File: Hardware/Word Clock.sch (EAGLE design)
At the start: 41 parts, among them IC1 MEGA32-A, IC2 HT7333, IC3 DS3231, IC4 MCP73831, J1 LiPo

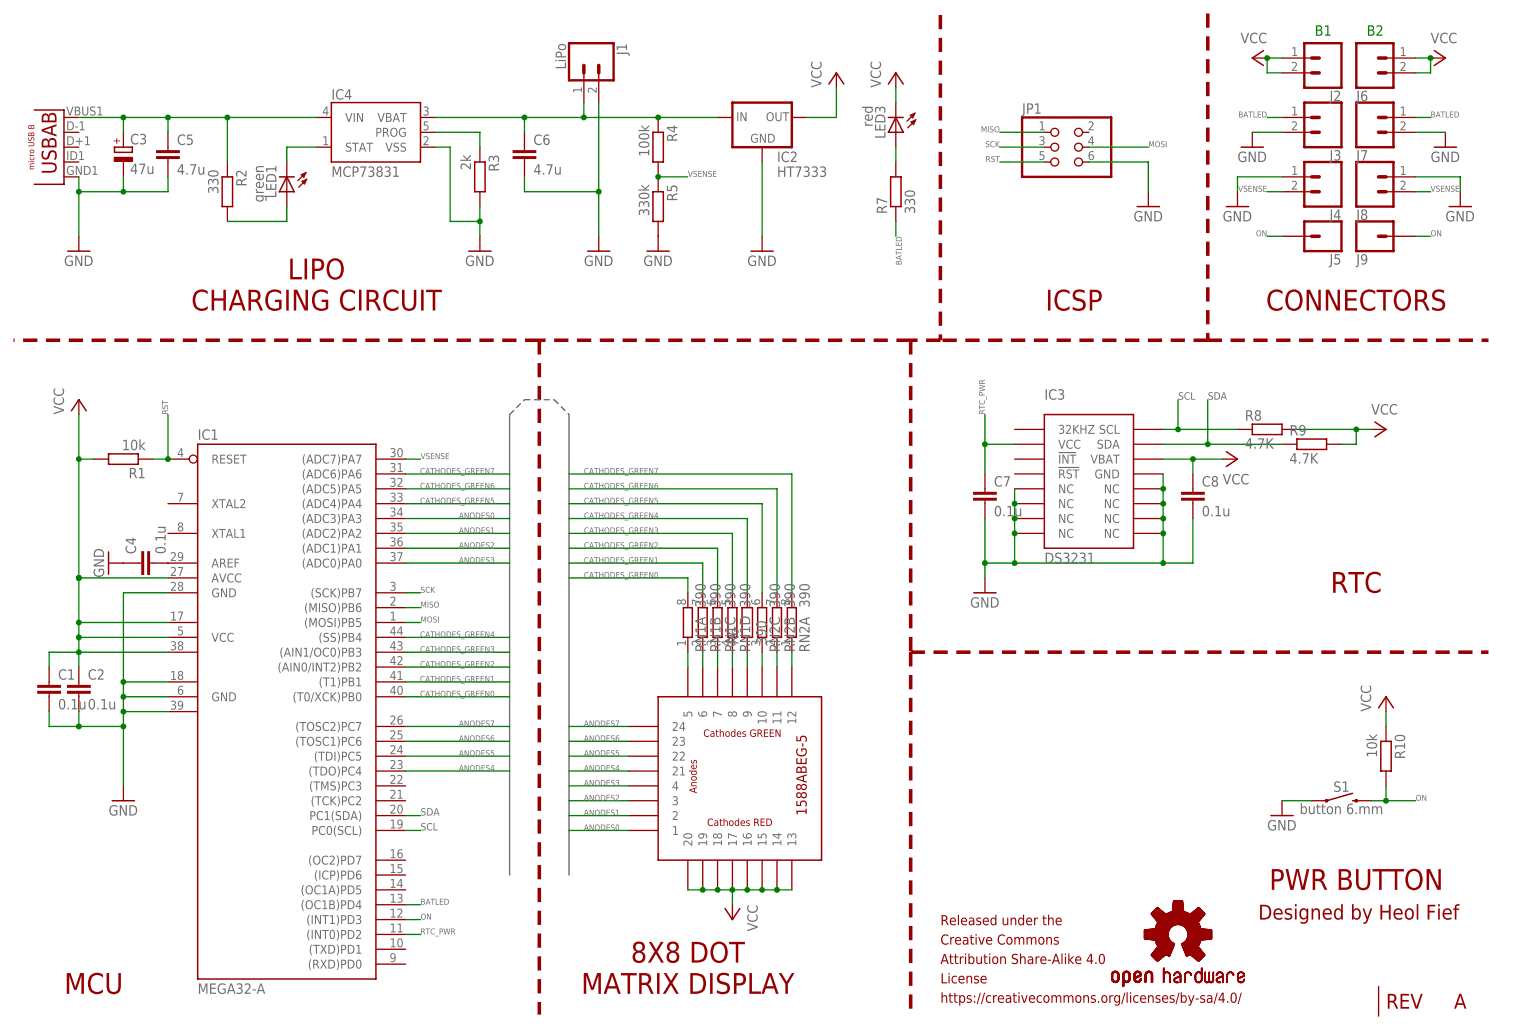
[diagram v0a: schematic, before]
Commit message: Update Eagle files
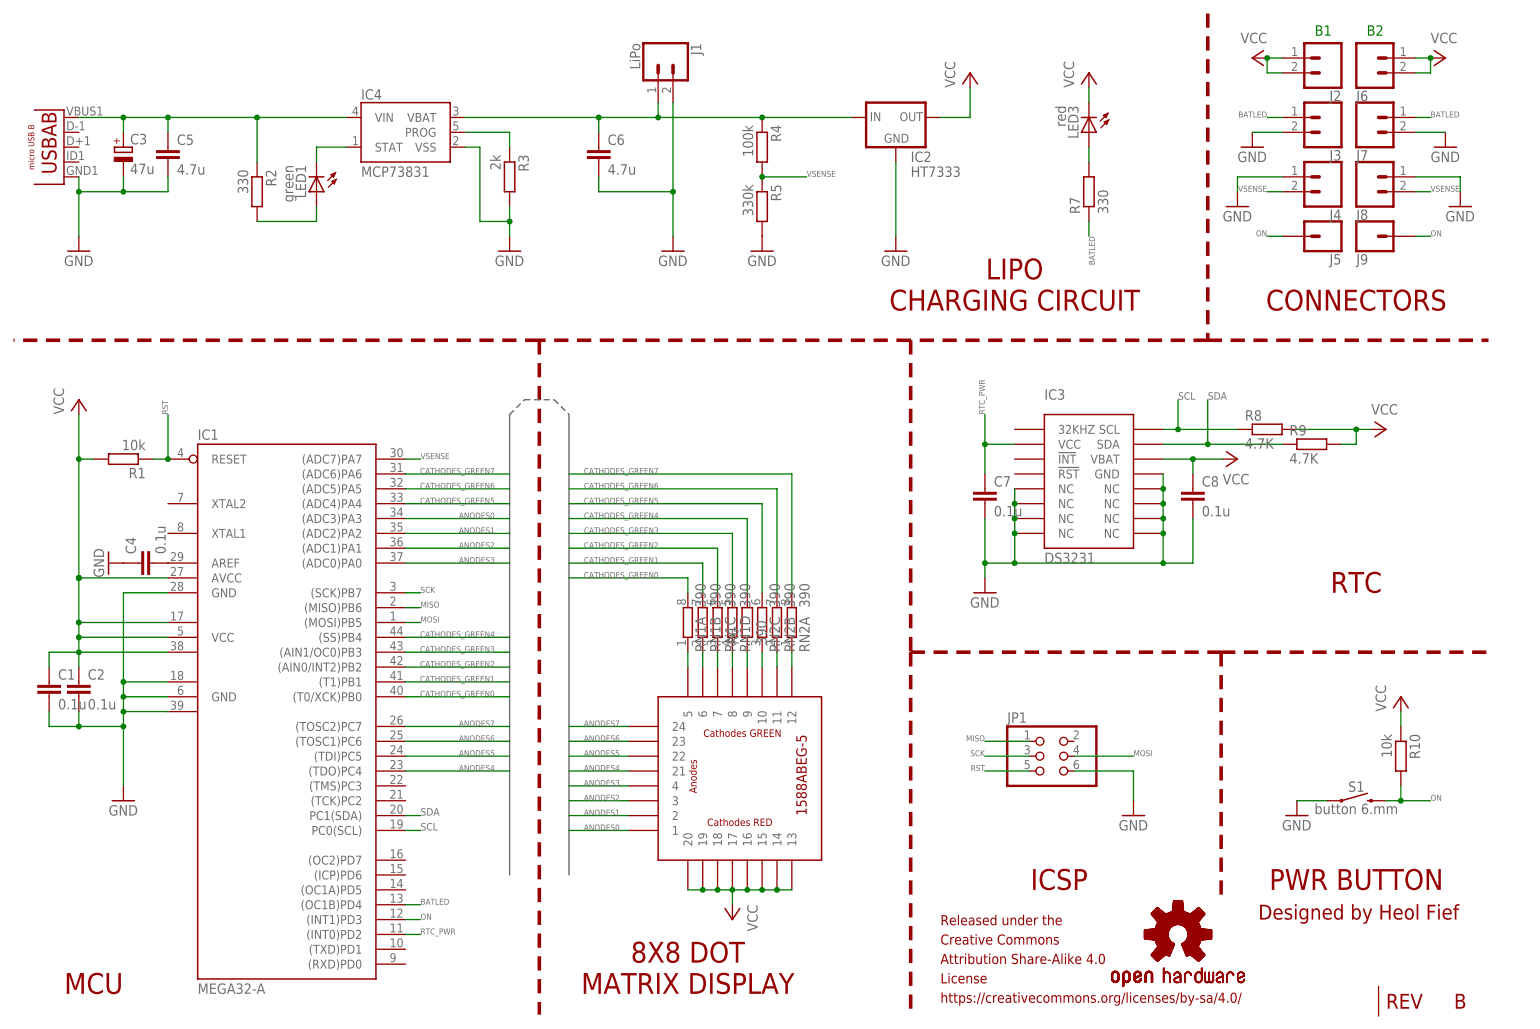
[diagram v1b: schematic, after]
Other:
- note added: "B"
- note removed: "A"
- moved on the sheet: C6, IC2, IC4, J1, JP1, LED1, LED3, R10, R2, R3, R4, R5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
